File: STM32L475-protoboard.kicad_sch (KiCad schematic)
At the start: 67 parts, among them J1 USB_HEADER, J10 Conn_01x02_Male, J11 SD_Card, J2 USB_B_Micro, J3 DCin, J4 STLINK, J5 W5500_ETHERNET, J6 STLINK2, J7 BOOT_MODE, J8 Conn_02x20_Odd_Even, J9 Conn_01x02_Male, SW1 RESET, U1 SRV05-4, U2 AMS1117-3.3, U3 STM32L475RCTx, Y1 Crystal_GND24, Y2 32.768k

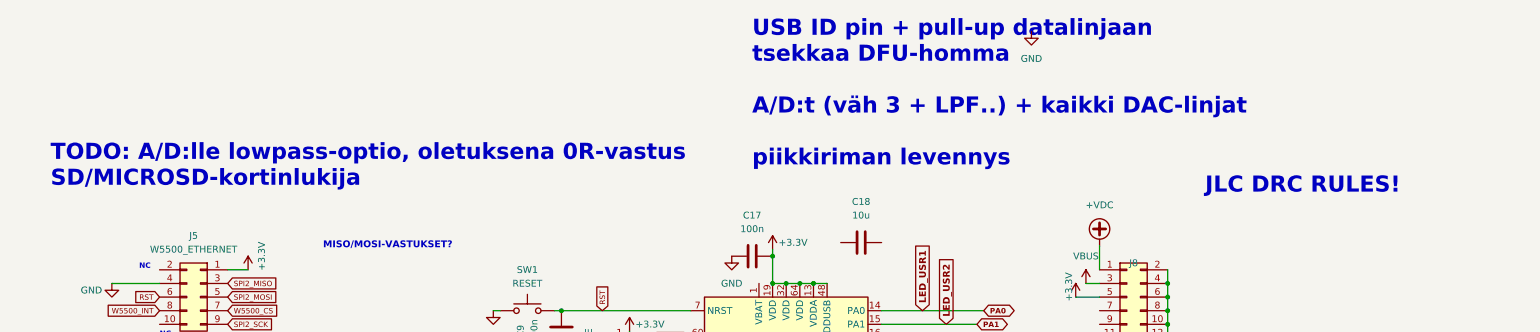
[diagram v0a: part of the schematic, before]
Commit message: todo update
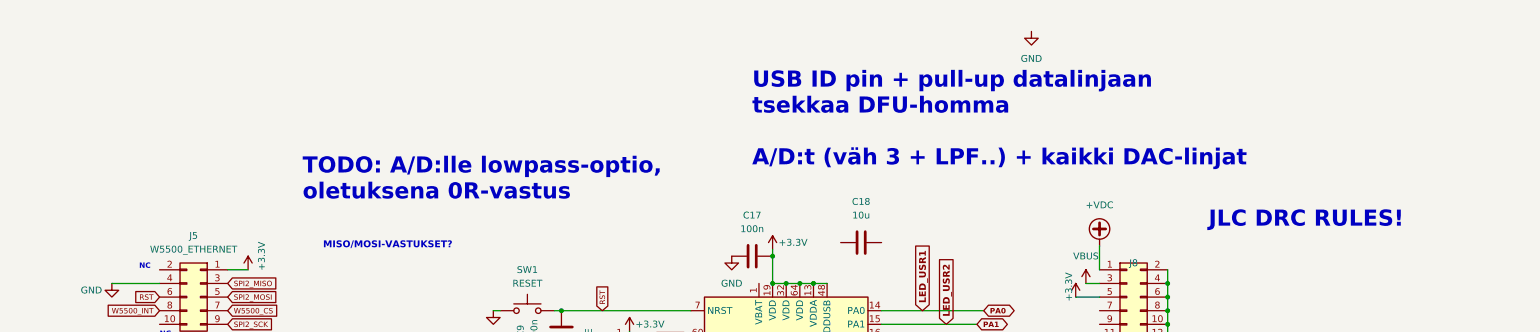
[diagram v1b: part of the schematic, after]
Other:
- note added: "TODO: A/D:lle lowpass-optio, oletuksena 0R-vastus"
- note added: "USB ID pin + pull-up datalinjaan tsekkaa DFU-homma A/D:t (väh 3 + LPF..) + kaikki DAC-linjat"
- note removed: "TODO: A/D:lle lowpass-optio, oletuksena 0R-vastus SD/MICROSD-kortinlukija"
- note removed: "USB ID pin + pull-up datalinjaan tsekkaa DFU-homma A/D:t (väh 3 + LPF..) + kaikki DAC-linjat piikkiriman levennys"
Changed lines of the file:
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@@
     (stroke (width 0) (type default) (color 0 0 0 0))
   )
-  (text "JLC DRC RULES!" (at 240.665 22.86 0)
+  (text "JLC DRC RULES!" (at 241.3 29.21 0)
     (effects (font (size 3 3) (thickness 0.6) bold) (justify left bottom))
   )
@@
     (effects (font (size 2 2) (thickness 0.254) bold) (justify left bottom))
   )
-  (text "USB ID pin + pull-up datalinjaan \ntsekkaa DFU-homma\n\nA/D:t (väh 3 + LPF..) + kaikki DAC-linjat\n\npiikkiriman levennys"
+  (text "USB ID pin + pull-up datalinjaan \ntsekkaa DFU-homma\n\nA/D:t (väh 3 + LPF..) + kaikki DAC-linjat\n"
     (at 156.21 17.78 0)
     (effects (font (size 3 3) (thickness 0.6) bold) (justify left bottom))
@@
     (effects (font (size 1.27 1.27)) (justify left bottom))
   )
-  (text "TODO: A/D:lle lowpass-optio, oletuksena 0R-vastus\nSD/MICROSD-kortinlukija"
-    (at 25.4 21.59 0)
+  (text "TODO: A/D:lle lowpass-optio, \noletuksena 0R-vastus"
+    (at 72.39 24.13 0)
     (effects (font (size 3 3) (thickness 0.6) bold) (justify left bottom))
   )
